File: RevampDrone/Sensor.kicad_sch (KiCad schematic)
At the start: 4 parts, among them U4 LSM6DSL, U5 LSM6DSL, U7 ADXL343, U9 BME280

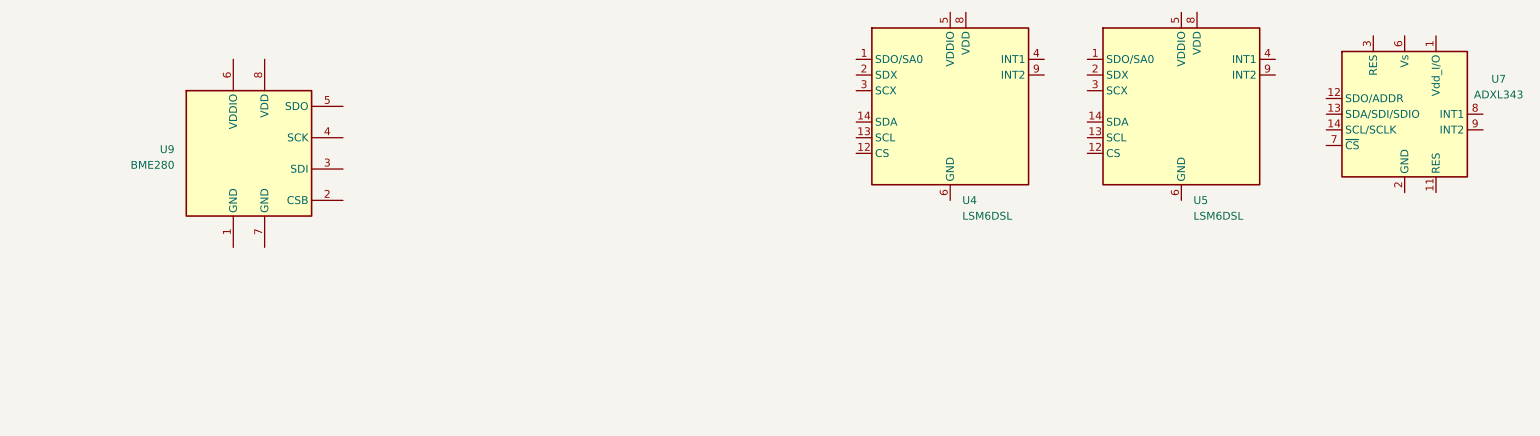
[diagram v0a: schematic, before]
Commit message: Get it on V7
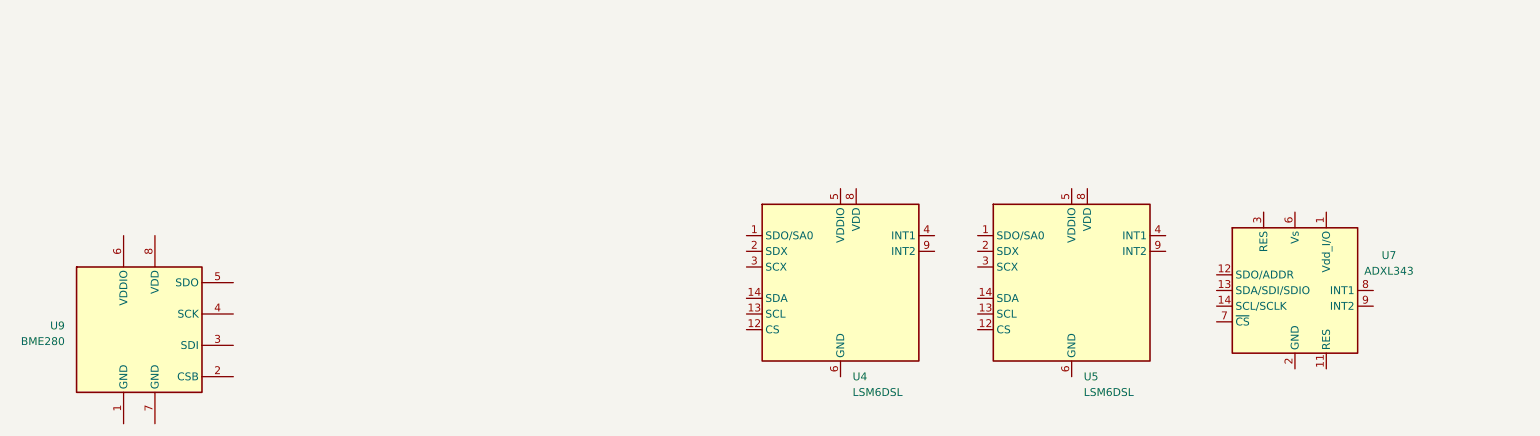
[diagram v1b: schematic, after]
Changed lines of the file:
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@@
 (kicad_sch (version 20230121) (generator eeschema)
   (paper "A4")
-  (symbol (lib_id "Sensor_Motion:LSM6DSL") (at 186.055 54.61 0) (unit 1)
+  (symbol (lib_id "Sensor:BME280") (at 54.61 90.805 0) (unit 1)
     (in_bom yes) (on_board yes) (dnp no) (fields_autoplaced)
-    (property "Reference" "U4" (at 188.0109 69.85 0)
+    (property "Reference" "U9" (at 42.545 90.17 0)
+      (effects (font (size 1.27 1.27)) (justify right))
+    )
+    (property "Value" "BME280" (at 42.545 92.71 0)
+      (effects (font (size 1.27 1.27)) (justify right))
+    )
+    (property "Footprint" "Package_LGA:Bosch_LGA-8_2.5x2.5mm_P0.65mm_ClockwisePinNumbering" (at 92.71 102.235 0)
+      (effects (font (size 1.27 1.27)) hide)
+    )
+    (property "Datasheet" "https://www.bosch-sensortec.com/media/boschsensortec/downloads/datasheets/bst-bme280-ds002.pdf" (at 54.61 95.885 0)
+      (effects (font (size 1.27 1.27)) hide)
+    )
+    (pin "1")
+    (pin "2")
+    (pin "3")
+    (pin "4")
+    (pin "5")
+    (pin "6")
+    (pin "7")
+    (pin "8")
+    (instances
+      (project "Sensors"
+        (path "/5830ddd2-2bd0-41fe-9aff-f385a123e2d6"
+          (reference "U9") (unit 1)
+        )
+      )
+      (project "RevampDrone"
+        (path "/a57dd8a7-b3ae-4be1-9fc6-9c9c7e0e2ba9/72301d20-d4dc-4e49-a22f-3d444c581bbe"
+          (reference "U9") (unit 1)
+        )
+      )
+      (project "DroneRevamp"
+        (path "/b197cc17-7ac5-409f-9705-26347f5a482b/cd60092a-1d91-439d-a55b-26434dc4780f"
+          (reference "U9") (unit 1)
+        )
+        (path "/b197cc17-7ac5-409f-9705-26347f5a482b/36d7dbc6-b6af-4bac-95b7-54c84bd2b8b3"
+          (reference "U9") (unit 1)
+        )
+      )
+    )
+  )
+  (symbol (lib_id "Sensor_Motion:LSM6DSL") (at 205.74 83.185 0) (unit 1)
+    (in_bom yes) (on_board yes) (dnp no) (fields_autoplaced)
+    (property "Reference" "U5" (at 207.6959 98.425 0)
       (effects (font (size 1.27 1.27)) (justify left))
     )
-    (property "Value" "LSM6DSL" (at 188.0109 72.39 0)
+    (property "Value" "LSM6DSL" (at 207.6959 100.965 0)
       (effects (font (size 1.27 1.27)) (justify left))
     )
-    (property "Footprint" "Package_LGA:LGA-14_3x2.5mm_P0.5mm_LayoutBorder3x4y" (at 175.895 72.39 0)
+    (property "Footprint" "Package_LGA:LGA-14_3x2.5mm_P0.5mm_LayoutBorder3x4y" (at 195.58 100.965 0)
       (effects (font (size 1.27 1.27)) (justify left) hide)
     )
-    (property "Datasheet" "https://www.st.com/resource/en/datasheet/lsm6dsl.pdf" (at 188.595 71.12 0)
+    (property "Datasheet" "https://www.st.com/resource/en/datasheet/lsm6dsl.pdf" (at 208.28 99.695 0)
       (effects (font (size 1.27 1.27)) hide)
     )
@@
     (pin "9")
     (instances
+      (project "Sensors"
+        (path "/5830ddd2-2bd0-41fe-9aff-f385a123e2d6"
+          (reference "U5") (unit 1)
+        )
+      )
+      (project "RevampDrone"
+        (path "/a57dd8a7-b3ae-4be1-9fc6-9c9c7e0e2ba9/72301d20-d4dc-4e49-a22f-3d444c581bbe"
+          (reference "U5") (unit 1)
+        )
+      )
       (project "DroneRevamp"
         (path "/b197cc17-7ac5-409f-9705-26347f5a482b/cd60092a-1d91-439d-a55b-26434dc4780f"
-          (reference "U4") (unit 1)
+          (reference "U5") (unit 1)
         )
         (path "/b197cc17-7ac5-409f-9705-26347f5a482b/36d7dbc6-b6af-4bac-95b7-54c84bd2b8b3"
-          (reference "U5") (unit 1)
+          (reference "U7") (unit 1)
         )
       )
     )
   )
-  (symbol (lib_id "Sensor_Motion:ADXL343") (at 259.715 55.88 0) (unit 1)
+  (symbol (lib_id "Sensor_Motion:ADXL343") (at 241.935 84.455 0) (unit 1)
     (in_bom yes) (on_board yes) (dnp no) (fields_autoplaced)
-    (property "Reference" "U7" (at 274.955 50.1903 0)
+    (property "Reference" "U7" (at 257.175 78.7653 0)
       (effects (font (size 1.27 1.27)))
     )
-    (property "Value" "ADXL343" (at 274.955 52.7303 0)
+    (property "Value" "ADXL343" (at 257.175 81.3053 0)
       (effects (font (size 1.27 1.27)))
     )
-    (property "Footprint" "Package_LGA:LGA-14_3x5mm_P0.8mm_LayoutBorder1x6y" (at 259.715 55.88 0)
+    (property "Footprint" "Package_LGA:LGA-14_3x5mm_P0.8mm_LayoutBorder1x6y" (at 241.935 84.455 0)
       (effects (font (size 1.27 1.27)) hide)
     )
-    (property "Datasheet" "https://www.analog.com/media/en/technical-documentation/data-sheets/ADXL343.pdf" (at 259.715 55.88 0)
+    (property "Datasheet" "https://www.analog.com/media/en/technical-documentation/data-sheets/ADXL343.pdf" (at 241.935 84.455 0)
       (effects (font (size 1.27 1.27)) hide)
     )
@@
     (pin "9")
     (instances
+      (project "Sensors"
+        (path "/5830ddd2-2bd0-41fe-9aff-f385a123e2d6"
+          (reference "U7") (unit 1)
+        )
+      )
+      (project "RevampDrone"
+        (path "/a57dd8a7-b3ae-4be1-9fc6-9c9c7e0e2ba9/72301d20-d4dc-4e49-a22f-3d444c581bbe"
+          (reference "U7") (unit 1)
+        )
+      )
       (project "DroneRevamp"
         (path "/b197cc17-7ac5-409f-9705-26347f5a482b/cd60092a-1d91-439d-a55b-26434dc4780f"
@@
     )
   )
-  (symbol (lib_id "Sensor_Motion:LSM6DSL") (at 223.52 54.61 0) (unit 1)
+  (symbol (lib_id "Sensor_Motion:LSM6DSL") (at 168.275 83.185 0) (unit 1)
     (in_bom yes) (on_board yes) (dnp no) (fields_autoplaced)
-    (property "Reference" "U5" (at 225.4759 69.85 0)
+    (property "Reference" "U4" (at 170.2309 98.425 0)
       (effects (font (size 1.27 1.27)) (justify left))
     )
-    (property "Value" "LSM6DSL" (at 225.4759 72.39 0)
+    (property "Value" "LSM6DSL" (at 170.2309 100.965 0)
       (effects (font (size 1.27 1.27)) (justify left))
     )
-    (property "Footprint" "Package_LGA:LGA-14_3x2.5mm_P0.5mm_LayoutBorder3x4y" (at 213.36 72.39 0)
+    (property "Footprint" "Package_LGA:LGA-14_3x2.5mm_P0.5mm_LayoutBorder3x4y" (at 158.115 100.965 0)
       (effects (font (size 1.27 1.27)) (justify left) hide)
     )
-    (property "Datasheet" "https://www.st.com/resource/en/datasheet/lsm6dsl.pdf" (at 226.06 71.12 0)
+    (property "Datasheet" "https://www.st.com/resource/en/datasheet/lsm6dsl.pdf" (at 170.815 99.695 0)
       (effects (font (size 1.27 1.27)) hide)
     )
@@
     (pin "9")
     (instances
+      (project "Sensors"
+        (path "/5830ddd2-2bd0-41fe-9aff-f385a123e2d6"
+          (reference "U4") (unit 1)
+        )
+      )
+      (project "RevampDrone"
+        (path "/a57dd8a7-b3ae-4be1-9fc6-9c9c7e0e2ba9/72301d20-d4dc-4e49-a22f-3d444c581bbe"
+          (reference "U4") (unit 1)
+        )
+      )
       (project "DroneRevamp"
         (path "/b197cc17-7ac5-409f-9705-26347f5a482b/cd60092a-1d91-439d-a55b-26434dc4780f"
+          (reference "U4") (unit 1)
+        )
+        (path "/b197cc17-7ac5-409f-9705-26347f5a482b/36d7dbc6-b6af-4bac-95b7-54c84bd2b8b3"
           (reference "U5") (unit 1)
         )
-        (path "/b197cc17-7ac5-409f-9705-26347f5a482b/36d7dbc6-b6af-4bac-95b7-54c84bd2b8b3"
-          (reference "U7") (unit 1)
-        )
       )
-    )
-  )
-  (symbol (lib_id "Sensor:BME280") (at 72.39 62.23 0) (unit 1)
-    (in_bom yes) (on_board yes) (dnp no) (fields_autoplaced)
-    (property "Reference" "U9" (at 60.325 61.595 0)
-      (effects (font (size 1.27 1.27)) (justify right))
-    )
-    (property "Value" "BME280" (at 60.325 64.135 0)
-      (effects (font (size 1.27 1.27)) (justify right))
-    )
-    (property "Footprint" "Package_LGA:Bosch_LGA-8_2.5x2.5mm_P0.65mm_ClockwisePinNumbering" (at 110.49 73.66 0)
-      (effects (font (size 1.27 1.27)) hide)
-    )
-    (property "Datasheet" "https://www.bosch-sensortec.com/media/boschsensortec/downloads/datasheets/bst-bme280-ds002.pdf" (at 72.39 67.31 0)
-      (effects (font (size 1.27 1.27)) hide)
-    )
-    (pin "1")
-    (pin "2")
-    (pin "3")
-    (pin "4")
-    (pin "5")
-    (pin "6")
-    (pin "7")
-    (pin "8")
-    (instances
-      (project "DroneRevamp"
-        (path "/b197cc17-7ac5-409f-9705-26347f5a482b/cd60092a-1d91-439d-a55b-26434dc4780f"
-          (reference "U9") (unit 1)
-        )
-        (path "/b197cc17-7ac5-409f-9705-26347f5a482b/36d7dbc6-b6af-4bac-95b7-54c84bd2b8b3"
-          (reference "U9") (unit 1)
-        )
-      )
